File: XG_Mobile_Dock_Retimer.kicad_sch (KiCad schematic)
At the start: 280 parts, among them J1 5-1775443-8, J13 39301240, J2 20455-040E-76, J3 20455-040E-76, J6 353180820, J7 CEE016400140111, J8 Retimer EEPROM, SW1 SW_Push, U1 DS160PT801ACBR, U2 TPS7A8400ARGRR, U7 TPS7A8400ARGRR

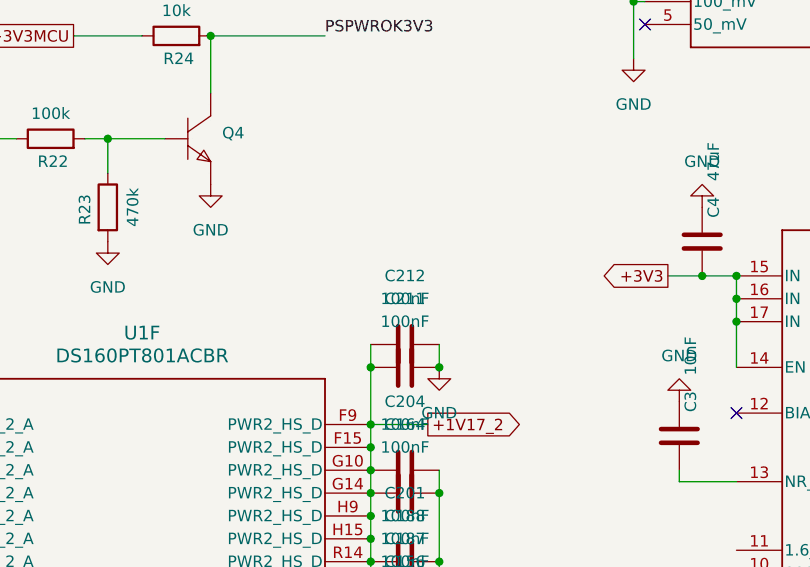
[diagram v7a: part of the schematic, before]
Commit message: eeeeeeeee
eeeeee
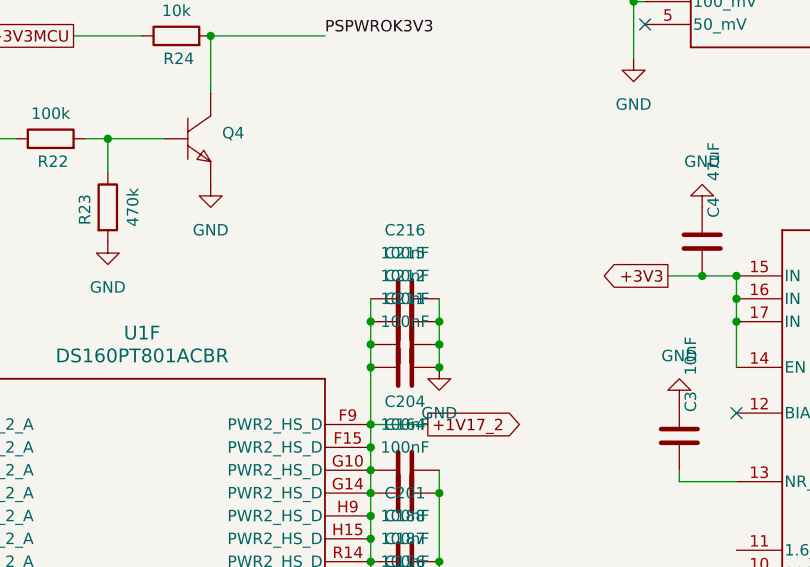
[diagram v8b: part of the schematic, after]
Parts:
- added C215, C216: 100nF, Capacitor_SMD:C_0201_0603Metric, symbol Device:C
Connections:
- net +1V17_2: now also C215.2, C216.2
- net GND: now also C215.1, C216.1
